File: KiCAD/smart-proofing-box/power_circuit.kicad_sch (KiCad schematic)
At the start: 0 parts

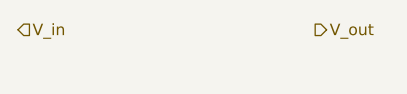
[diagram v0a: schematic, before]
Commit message: continued sketching rough design
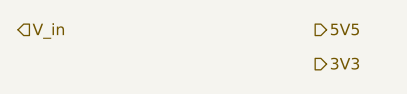
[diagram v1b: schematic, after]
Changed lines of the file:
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@@
 	(generator_version "8.0")
 	(paper "A4")
-	(hierarchical_label "V_out"
+	(hierarchical_label "3V3"
+		(shape output)
+		(at 74.93 90.17 0)
+		(fields_autoplaced yes)
+		(effects
+			(font
+				(size 1.27 1.27)
+			)
+			(justify left)
+		)
+	)
+	(hierarchical_label "5V5"
 		(shape output)
 		(at 74.93 86.36 0)
